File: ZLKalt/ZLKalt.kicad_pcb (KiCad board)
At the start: 2 copper layers, 88.8 x 45.5 mm, 30 parts, among them J1 Conn_02x04_Counter_Clockwise, J2 Conn_02x04_Counter_Clockwise, U1 AT90S1200A

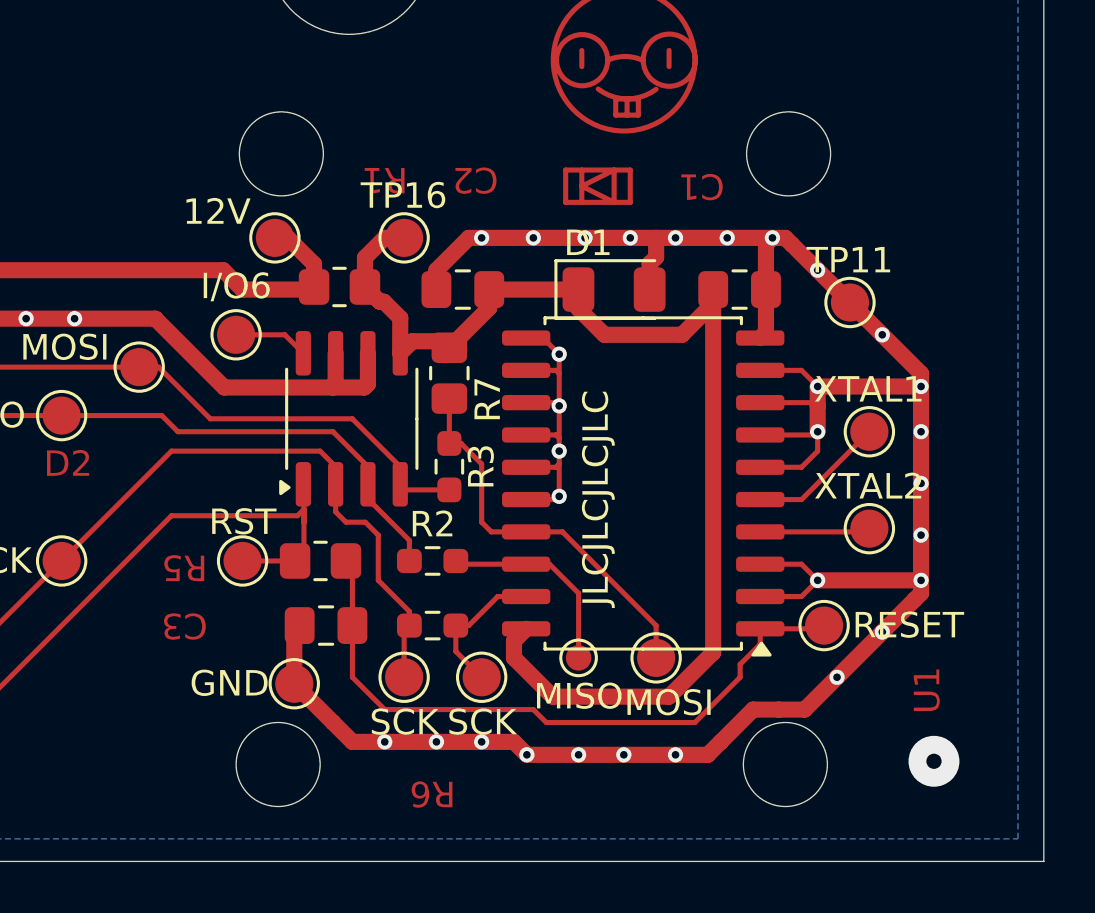
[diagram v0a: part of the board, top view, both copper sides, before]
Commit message: silkscreen, parts
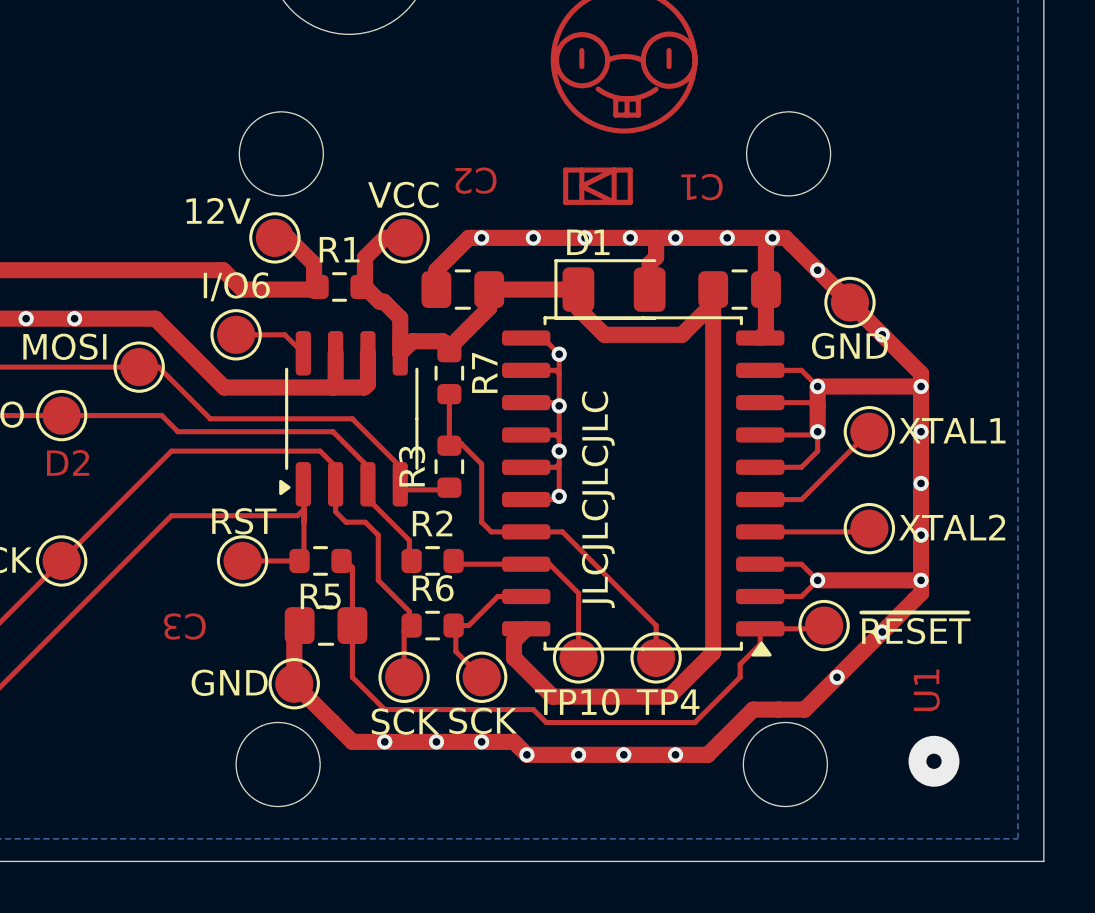
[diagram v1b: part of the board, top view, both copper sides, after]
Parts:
- C1, C2, C3: value C -> 100nF
- D1: value D -> 0,5W 4,7V
- D2: value ~ -> ESDA6V1U1
- R1: value R -> 270; footprint Resistor_SMD:R_0805_2012Metric_Pad1.20x1.40mm_HandSolder -> Resistor_SMD:R_0603_1608Metric
- R2, R6: value 4640 -> 4700; footprint Resistor_SMD:R_0603_1608Metric_Pad0.98x0.95mm_HandSolder -> Resistor_SMD:R_0603_1608Metric
- R3: value R -> 4700; footprint Resistor_SMD:R_0603_1608Metric_Pad0.98x0.95mm_HandSolder -> Resistor_SMD:R_0603_1608Metric
- R5, R7: footprint Resistor_SMD:R_0805_2012Metric_Pad1.20x1.40mm_HandSolder -> Resistor_SMD:R_0603_1608Metric
- TP10: renamed from MISO; footprint TestPoint:TestPoint_Pad_D1.0mm -> TestPoint:TestPoint_Pad_D1.5mm
- renumbered SCK to TP12, RESET to TP13, XTAL1 to TP14, XTAL2 to TP15, MOSI to TP4, SCK to TP6

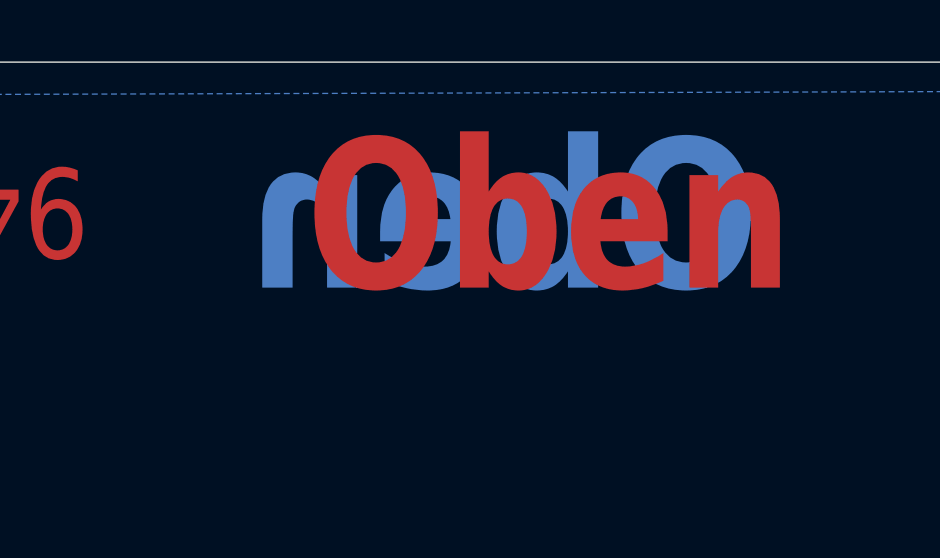
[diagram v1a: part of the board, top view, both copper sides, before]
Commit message: aussparung
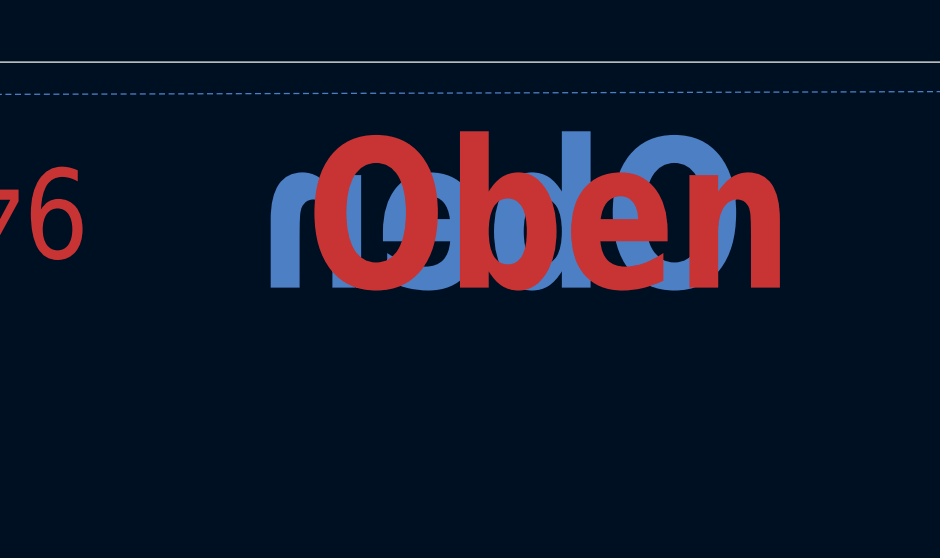
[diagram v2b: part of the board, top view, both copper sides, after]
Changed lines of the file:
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@@
 	)
 	(gr_text "Oben"
-		(at 101.092 39.497 -0)
+		(at 100.584 39.497 0)
 		(layer "B.Cu")
 		(effects
 			(font
-				(size 5 4.2)
+				(size 5 4)
 				(thickness 0.3)
 				(bold yes)
@@
 	)
 	(zone
+		(net 0)
+		(net_name "")
+		(layer "B.Cu")
+		(hatch edge 0.5)
+		(connect_pads
+			(clearance 0)
+		)
+		(min_thickness 0.25)
+		(filled_areas_thickness no)
+		(keepout
+			(tracks allowed)
+			(vias allowed)
+			(pads allowed)
+			(copperpour not_allowed)
+			(footprints allowed)
+		)
+		(placement
+			(enabled no)
+			(sheetname "/")
+		)
+		(fill
+			(thermal_gap 0.5)
+			(thermal_bridge_width 0.5)
+		)
+		(polygon
+			(pts
+				(xy 84.328 40.64) (xy 101.854 40.64) (xy 101.854 31.496) (xy 84.328 31.496)
+			)
+		)
+	)
+	(zone
